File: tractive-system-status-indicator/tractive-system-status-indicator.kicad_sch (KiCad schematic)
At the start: 37 parts, among them J1 Conn_01x06

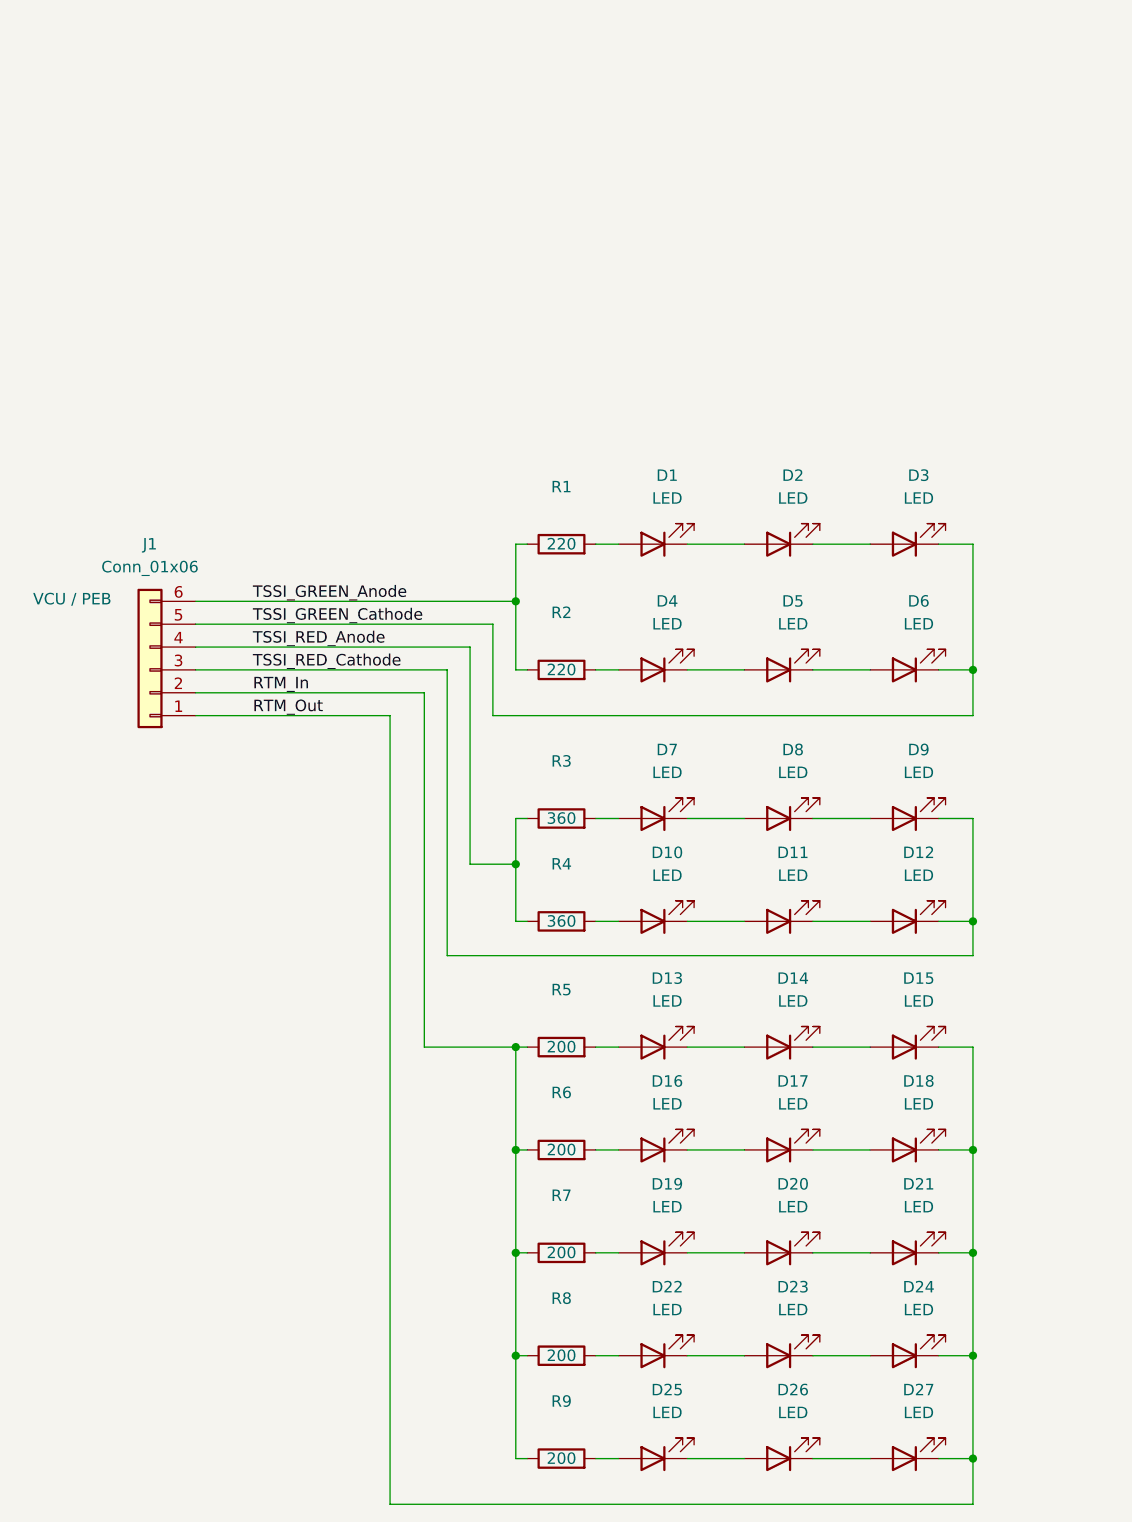
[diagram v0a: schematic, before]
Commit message: Updated template, resourced LED's,  placed components
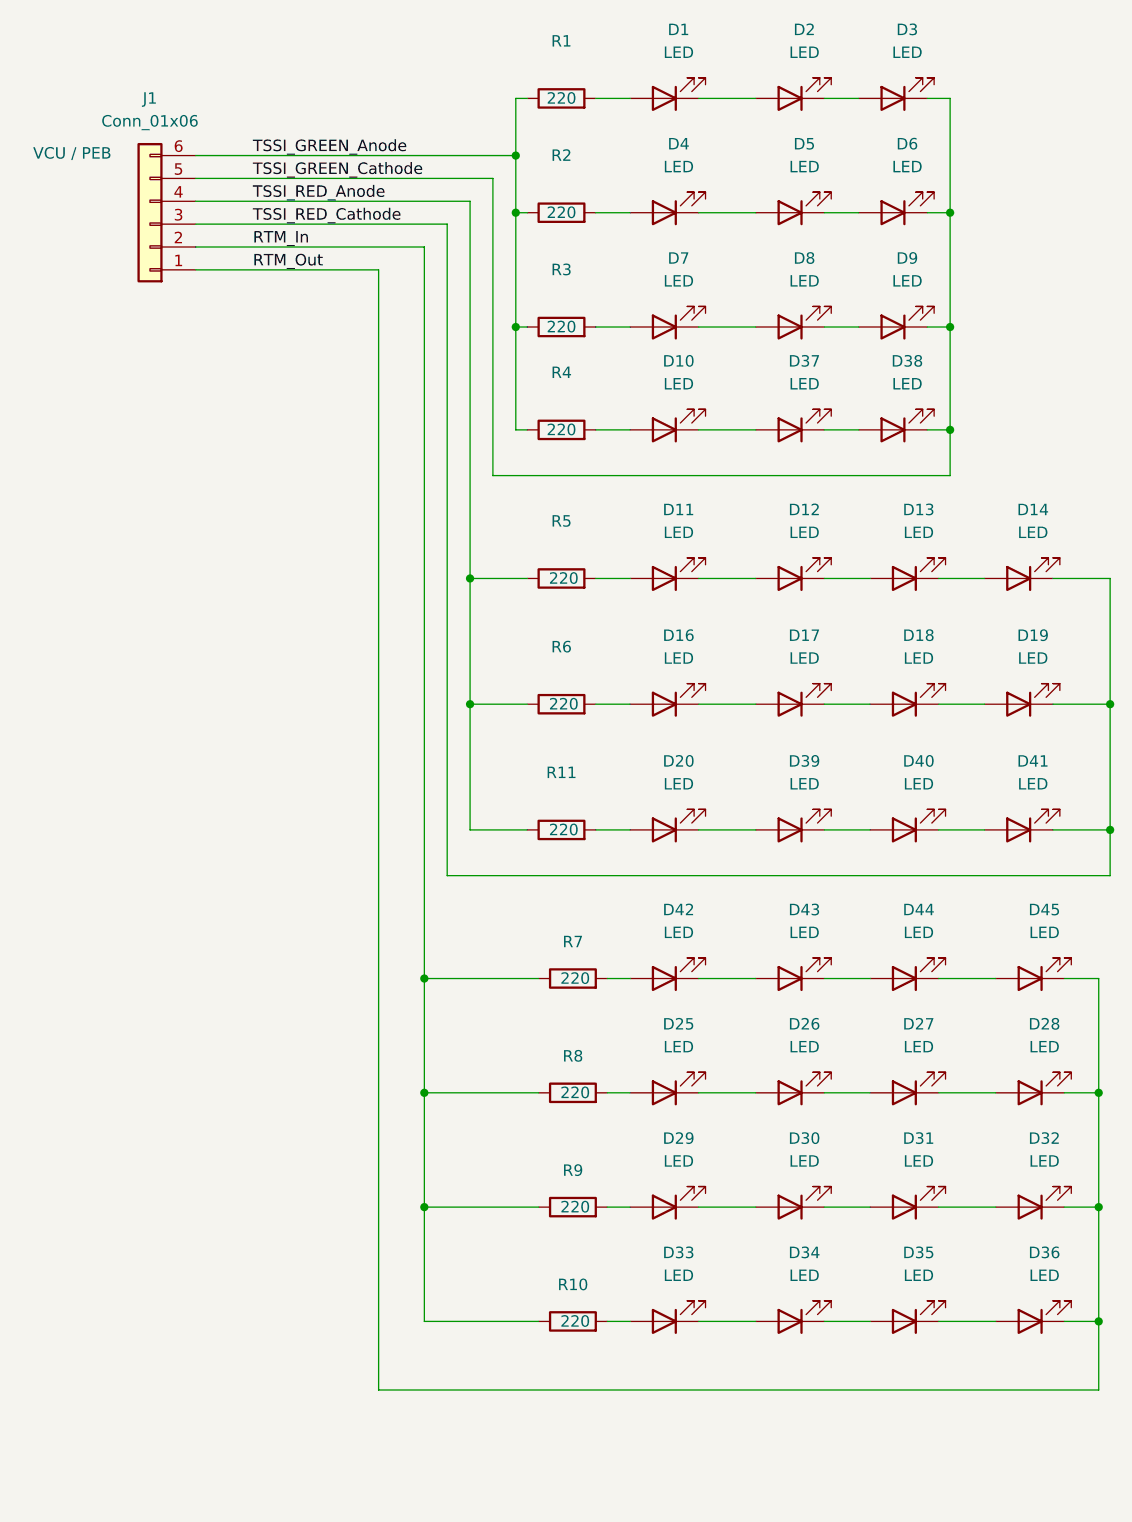
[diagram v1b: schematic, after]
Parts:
- removed D15, D21, D22, D23, D24: LED, LED_SMD:LED_0603_1608Metric_Pad1.05x0.95mm_HandSolder, symbol Device:LED
- added D28, D29, D30, D31, D32, D33, D34, D35, D36, D37, D38, D42, D43, D44, D45: LED, LED_SMD:LED_Avago_PLCC4_3.2x2.8mm_CW, symbol Device:LED
- added D39, D40, D41: LED, LED_SMD:LED_Everlight-SMD3528_3.5x2.8mm_67-21ST, symbol Device:LED
- added R10, R11: 220, Resistor_SMD:R_0603_1608Metric_Pad0.98x0.95mm_HandSolder, symbol Device:R
- D1, D10, D2, D3, D4, D5, D6, D7, D8, D9: footprint LED_SMD:LED_0805_2012Metric_Pad1.15x1.40mm_HandSolder -> LED_SMD:LED_Avago_PLCC4_3.2x2.8mm_CW; Digi URL https://www.digikey.com/en/products/detail/xinglight/XL-TD2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 -> (none)
- D11, D12: footprint LED_SMD:LED_0805_2012Metric_Pad1.15x1.40mm_HandSolder -> LED_SMD:LED_Everlight-SMD3528_3.5x2.8mm_67-21ST; Digi URL https://www.digikey.com/en/products/detail/xinglight/XL-TD2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 -> (none)
- D13, D14, D16, D17, D18, D19, D20: footprint LED_SMD:LED_0603_1608Metric_Pad1.05x0.95mm_HandSolder -> LED_SMD:LED_Everlight-SMD3528_3.5x2.8mm_67-21ST; Digi URL https://www.digikey.com/en/products/detail/ams-osram-usa-in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 -> (none)
- D25, D26, D27: footprint LED_SMD:LED_0603_1608Metric_Pad1.05x0.95mm_HandSolder -> LED_SMD:LED_Avago_PLCC4_3.2x2.8mm_CW; Digi URL https://www.digikey.com/en/products/detail/ams-osram-usa-in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 -> (none)
- R3, R4: value 360 -> 220
- R5, R6, R7, R8, R9: value 200 -> 220
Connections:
- net RTM_In: now also R10.1; no longer R5.1, R6.1
- net RTM_Out: now also D28.1 (K), D32.1 (K), D36.1 (K), D45.1 (K); no longer D18.1 (K), D27.1 (K)
- net TSSI_GREEN_Anode: now also R3.1, R4.1
- net TSSI_GREEN_Cathode: now also D9.1 (K), D38.1 (K)
- net TSSI_RED_Anode: now also R5.1, R6.1, R11.1; no longer R3.1, R4.1
- net TSSI_RED_Cathode: now also D14.1 (K), D19.1 (K), D41.1 (K); no longer D12.1 (K), D9.1 (K)
- net at D11.2 (A): now also R5.2; no longer D10.1 (K)
- net at D13.2 (A): now also D12.1 (K); no longer R5.2
- net at D20.2 (A): now also R11.2; no longer D19.1 (K)
- net at R7.2: now also D42.2 (A); no longer D19.2 (A)
- net at R8.2: now also D25.2 (A)
- net at R9.2: now also D29.2 (A); no longer D25.2 (A)
- net at D20.1 (K): now also D39.2 (A)
- new net: D40.1 (K), D41.2 (A)
- new net: D33.2 (A), R10.2
- new net: D30.1 (K), D31.2 (A)
- new net: D29.1 (K), D30.2 (A)
- new net: D34.1 (K), D35.2 (A)
- new net: D33.1 (K), D34.2 (A)
- new net: D39.1 (K), D40.2 (A)
- new net: D37.1 (K), D38.2 (A)
- new net: D10.1 (K), D37.2 (A)
- new net: D35.1 (K), D36.2 (A)
- new net: D18.1 (K), D19.2 (A)
- new net: D42.1 (K), D43.2 (A)
- new net: D44.1 (K), D45.2 (A)
- new net: D43.1 (K), D44.2 (A)
- new net: D27.1 (K), D28.2 (A)
- new net: D31.1 (K), D32.2 (A)
